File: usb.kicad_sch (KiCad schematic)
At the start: 80 parts, among them J1 USB_C_Receptacle_USB2.0, J2 USB_C_Receptacle_USB2.0, J3 USB_C_Receptacle_USB2.0, J4 USB_C_Receptacle_USB2.0, U1 MIMX8MM6DVTLZAA, U10 D5V0H1B2LP, U11 TPD4E02B04, U12 TPD4E02B04, U13 74LVC2G07, U14 D5V0H1B2LP, U15 CH343P, U16 TPD4E02B04, U17 INA231, U18 D5V0H1B2LP, U19 TS3USB221E, U20 TPD4E02B04, U4 74LVC2G04, U5 NX5P3363, U6 TUSB320LAI, U7 NX5P3363, U8 TUSB320LAI, U9 D5V0H1B2LP

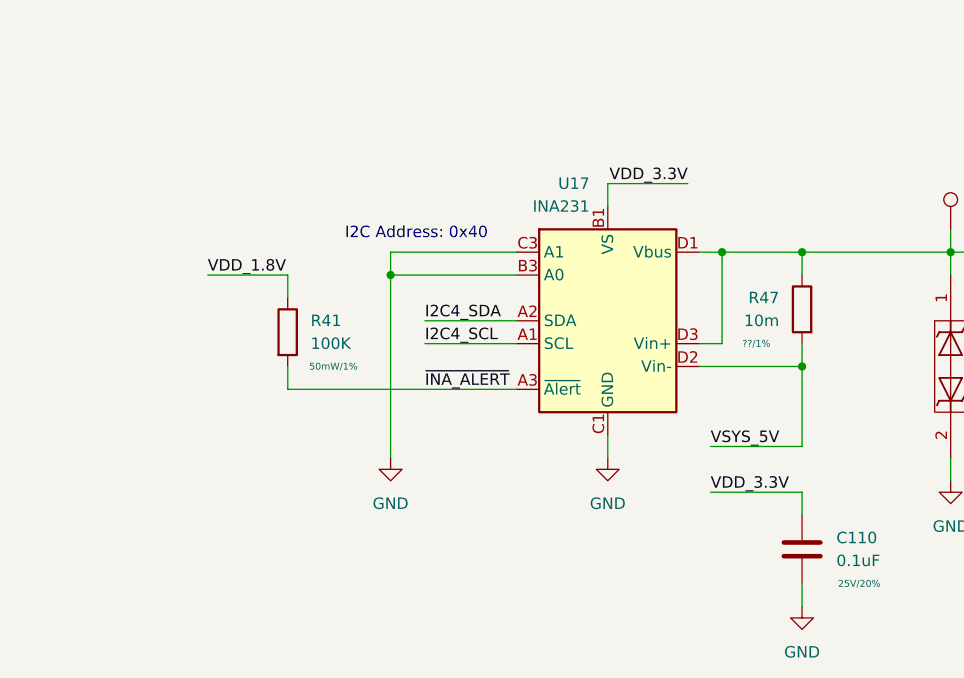
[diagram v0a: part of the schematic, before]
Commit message: pmic routing almost done
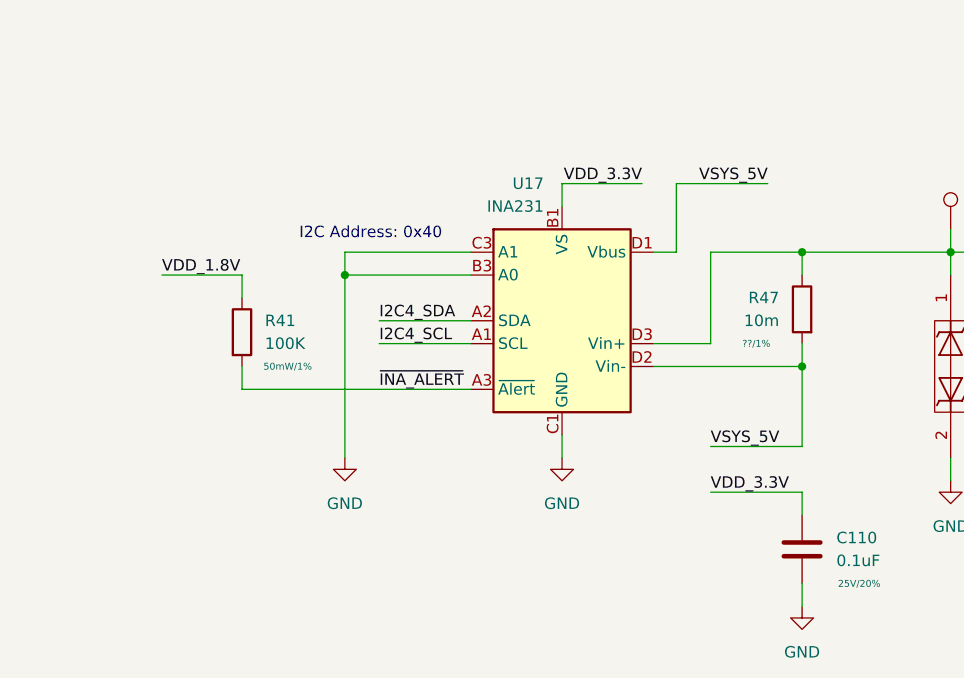
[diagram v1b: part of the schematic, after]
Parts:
- C102, C103: footprint Capacitor_SMD:C_0603_1608Metric -> qsbc:C_0603_1608Metric
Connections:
- net USB4_VBUS: no longer U17.D1 (Vbus)
- net VSYS_5V: now also U17.D1 (Vbus)
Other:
- moved on the sheet: R41, U17
